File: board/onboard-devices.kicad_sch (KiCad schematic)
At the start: 32 parts, among them Q1 DMG1012T, Q2 DMG1012T, Q3 DMG1012T, Q4 DMG1012T, SW1 SW_DIP_x08

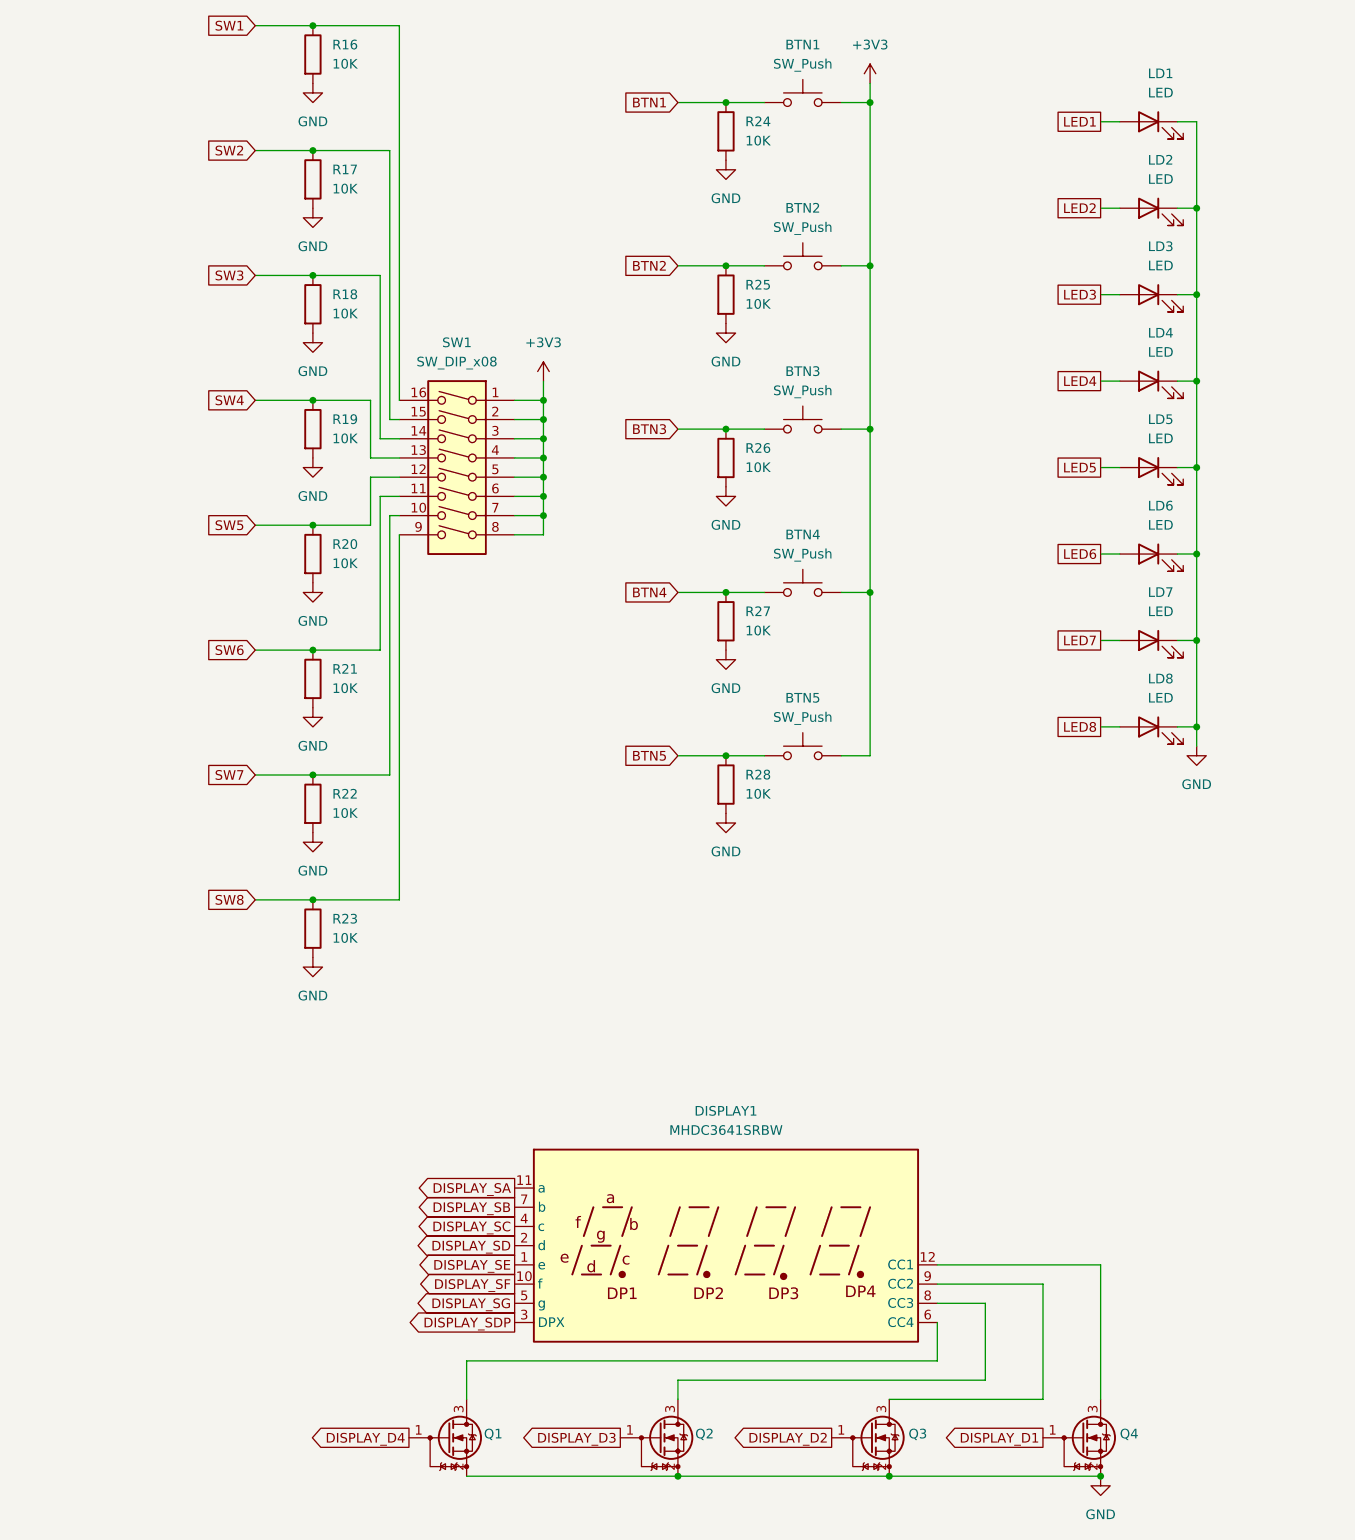
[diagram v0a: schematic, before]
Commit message: Change switches
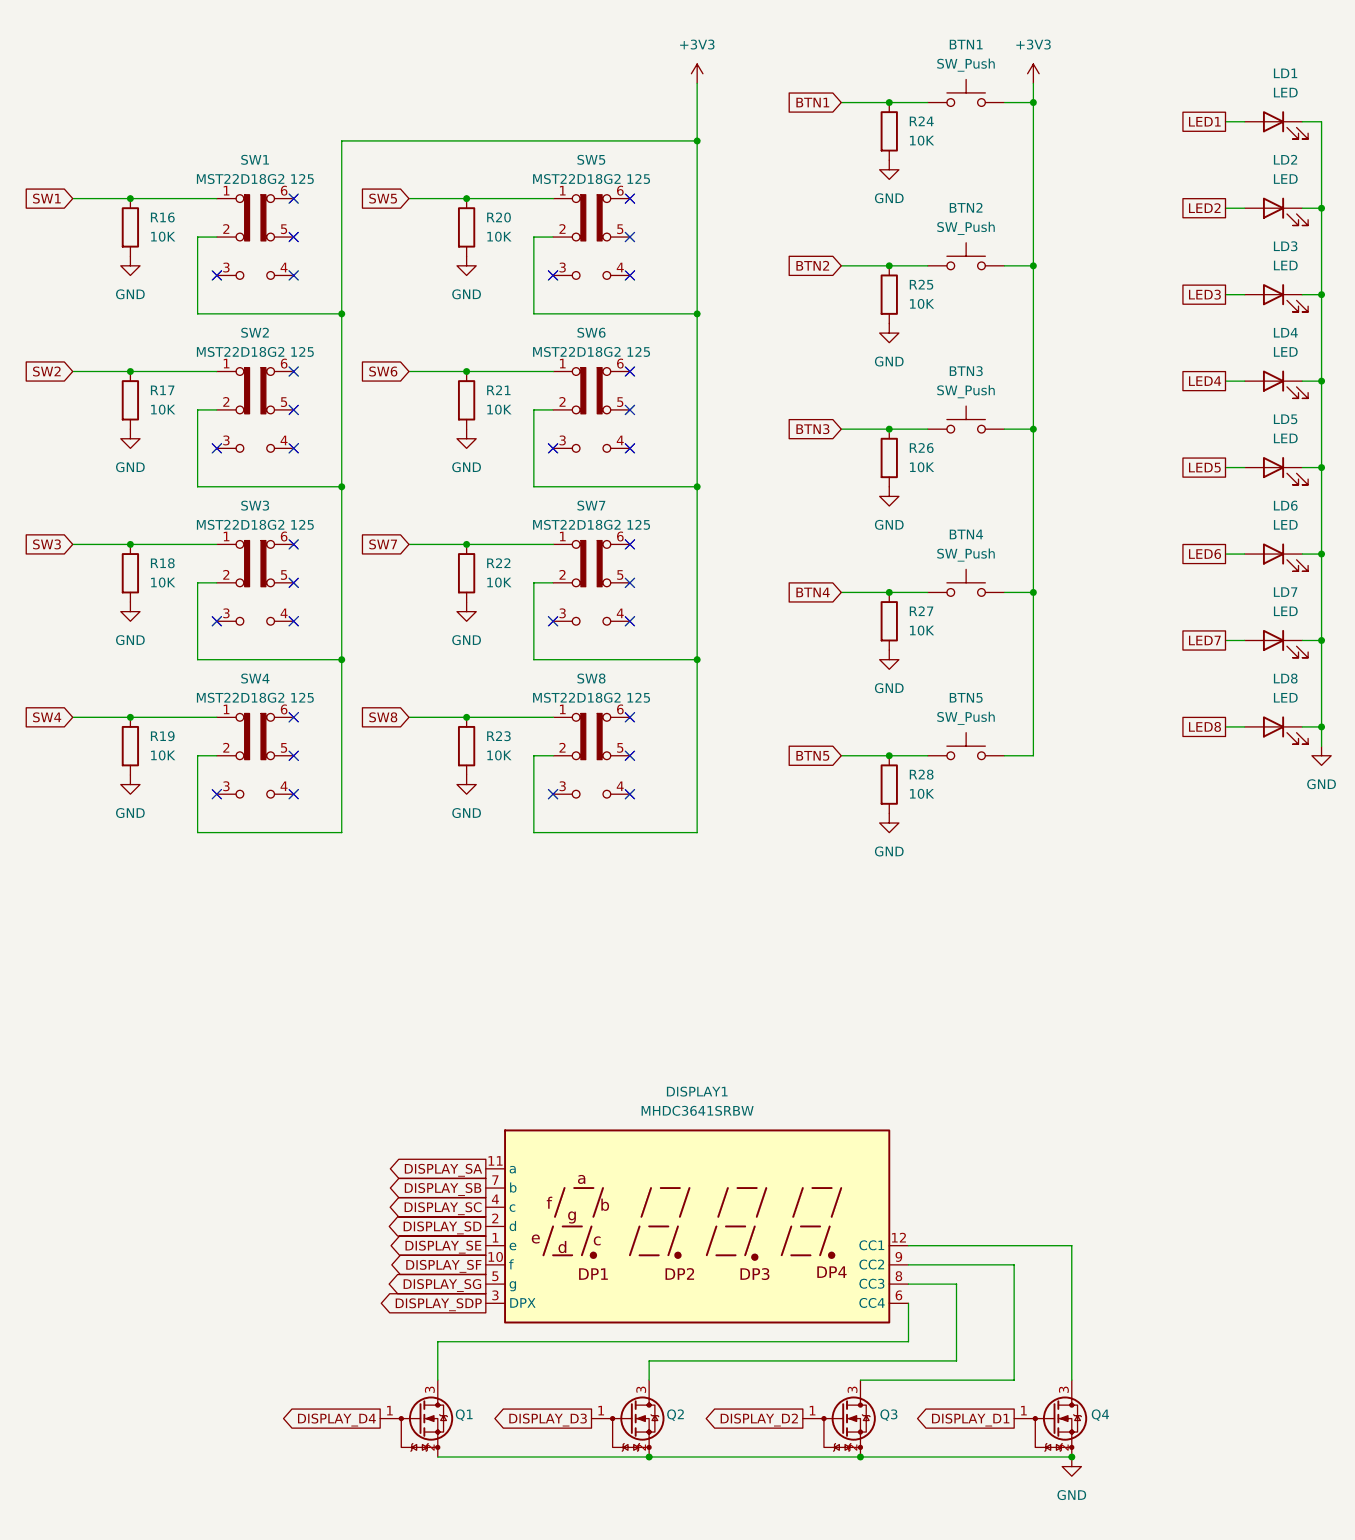
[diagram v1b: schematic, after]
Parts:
- removed SW1: SW_DIP_x08, Button_Switch_SMD:SW_DIP_SPSTx08_Slide_6.7x21.88mm_W6.73mm_P2.54mm_LowProfile_JPin, symbol Switch:SW_DIP_x08
- added SW1, SW2, SW3, SW4, SW5, SW6, SW7, SW8: MST22D18G2 125, HispalisFPGA:SW-SMD_MST22D18G2, symbol Switch:SW_Slide_DPDT
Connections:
- net +3V3: now also SW1.2 (B), SW2.2 (B), SW3.2 (B), SW4.2 (B), SW5.2 (B), SW6.2 (B), SW7.2 (B), SW8.2 (B)
- net SW1: now also SW1.1 (A)
- net SW2: now also SW2.1 (A)
- net SW3: now also SW3.1 (A)
- net SW4: now also SW4.1 (A)
- net SW5: now also SW5.1 (A)
- net SW6: now also SW6.1 (A)
- net SW7: now also SW7.1 (A)
- net SW8: now also SW8.1 (A)
- no-connect marks 0 -> 32
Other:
- moved on the sheet: BTN1, BTN2, BTN3, BTN4, BTN5, DISPLAY1, LD1, LD2, LD3, LD4, LD5, LD6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
